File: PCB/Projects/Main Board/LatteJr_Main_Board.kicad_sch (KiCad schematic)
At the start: 134 parts, among them IC1 BQ27621YZFR-G1A, J1 Conn_01x04_Pin, J3 USB4056-03-A, J4 Conn_01x04_Pin, J5 Conn_01x04_Pin, J6 Conn_01x02_Socket, P1 RPI-RM2, Q1 BSS138DW, Q2 BSS138DW, SW1 SW_Push, SW2 SW_Push, SW3 SW_Push, SW4 SW_Push, SW5 SW_Push, SW6 SW_Push, SW7 SW_Push, SW8 SW_Push, U1 RP2350_60QFN, U10 HAL4395, U11 HAL4395, U12 HAL4395, U13 HAL4395, U14 HAL4395, U15 HAL4395, U16 HAL4395, U2 HAL4395, U3 HAL4395, U4 TPS63001DRCR, U5 BQ25180, U6 USBLC6-2P6, U7 USBLC6-2P6, U8 USBLC6-2P6, U9 HAL4395, Y1 ABM8-272-T3

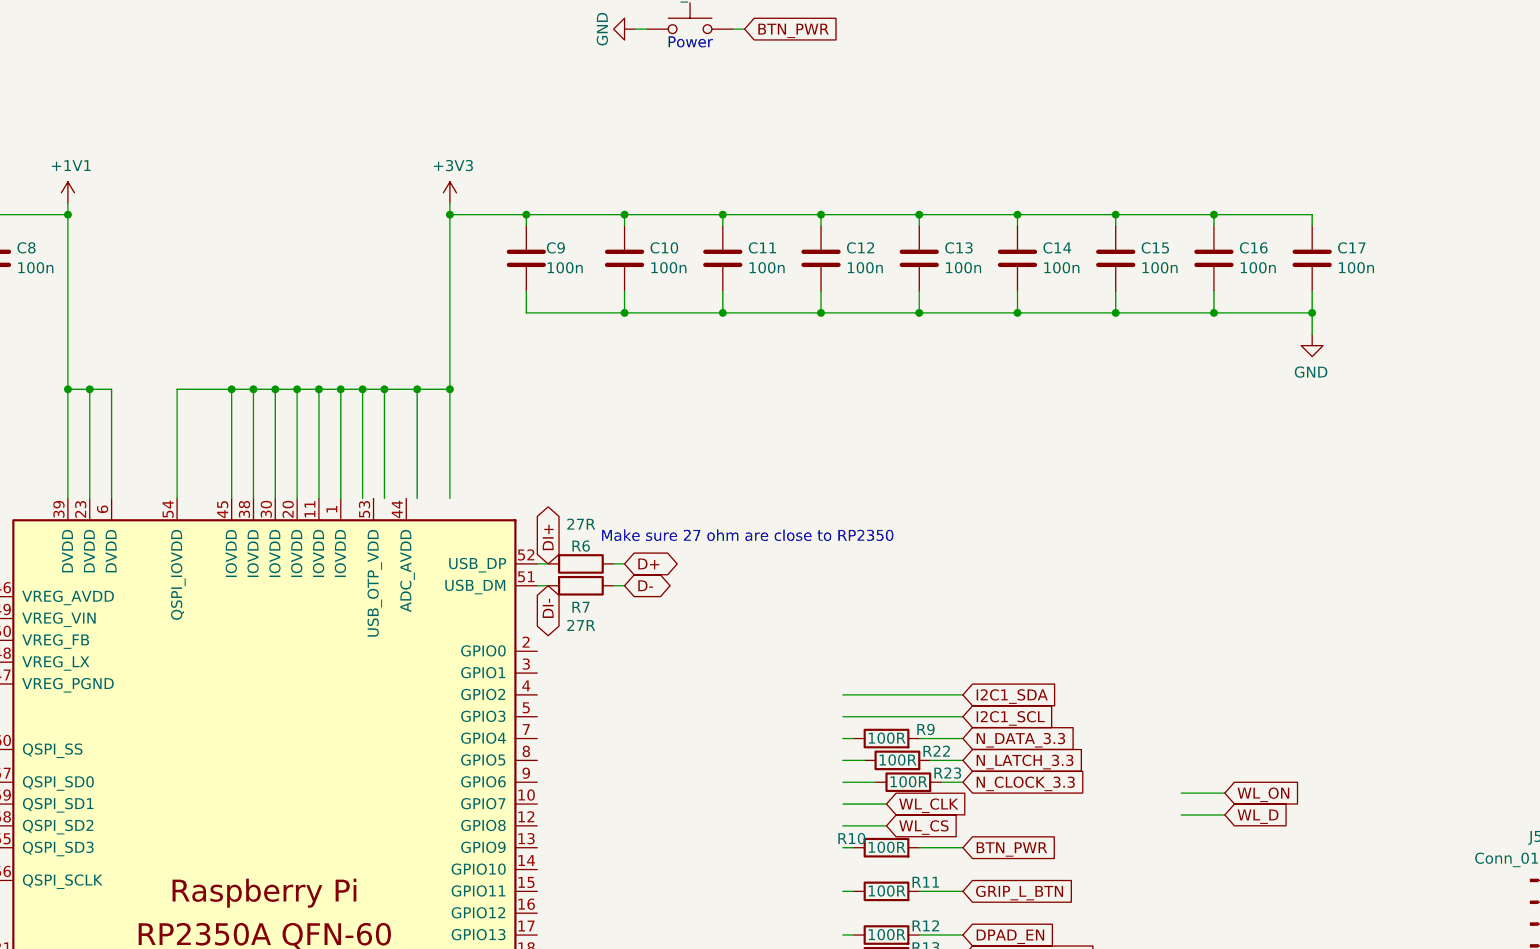
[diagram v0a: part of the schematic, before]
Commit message: Some Routing
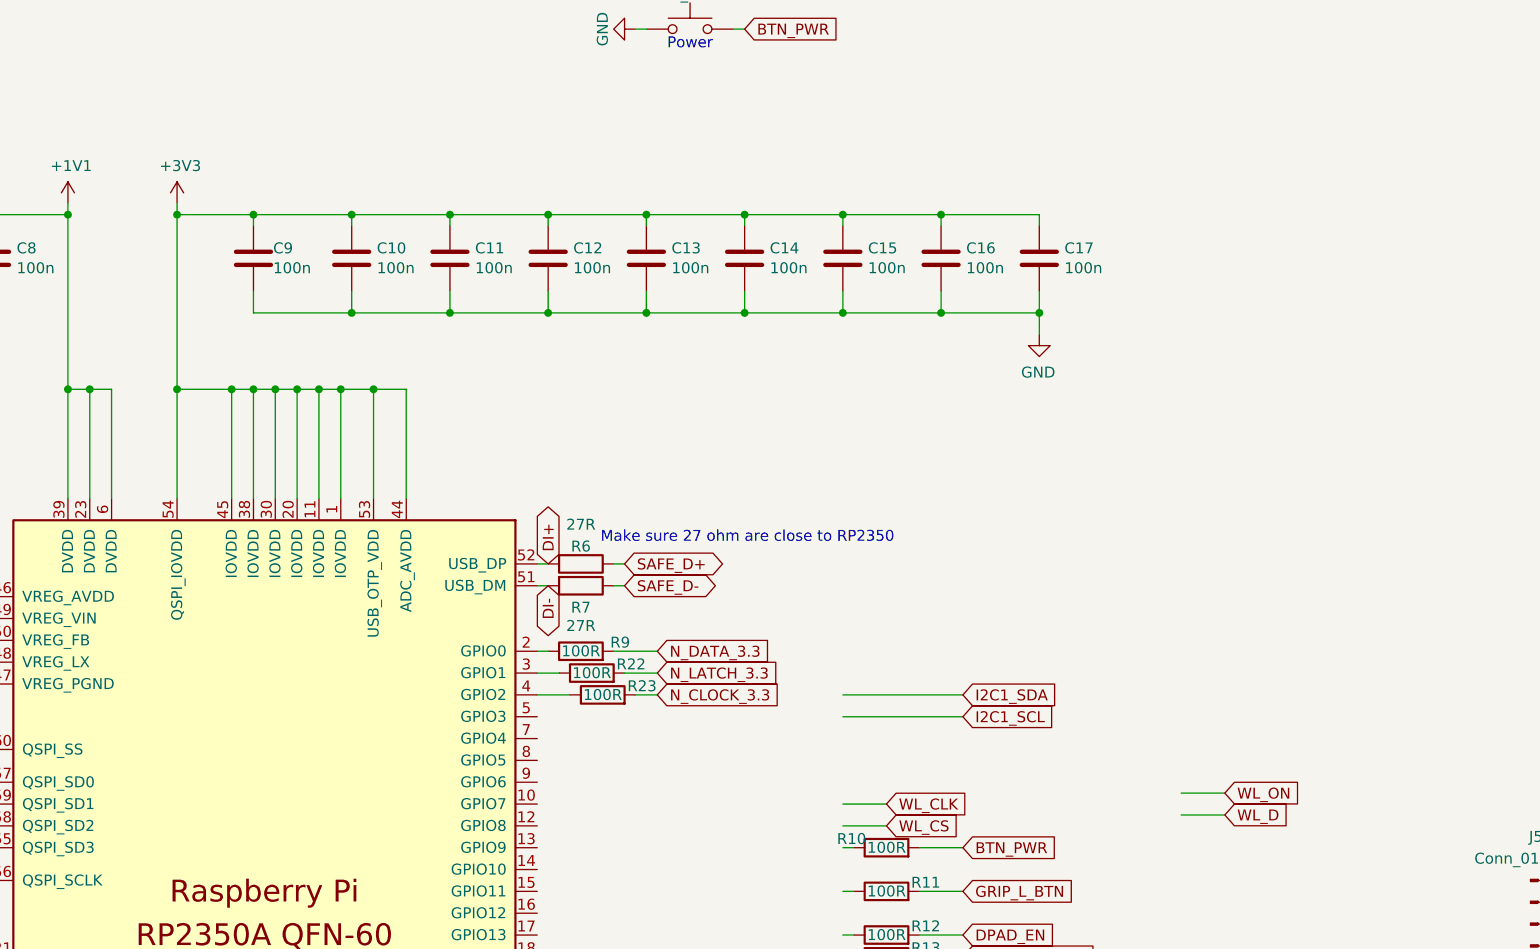
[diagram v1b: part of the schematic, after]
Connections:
- net +3V3: now also U1.44 (ADC_AVDD), U1.53 (USB_OTP_VDD)
- net D+: no longer R6.1
- net D-: no longer R7.1
- net SAFE_D+: now also R6.1
- net SAFE_D-: now also R7.1
- net at R22.1: now also U1.3 (GPIO1)
- net at R23.1: now also U1.4 (GPIO2)
- net at U1.2 (GPIO0): now also R9.1
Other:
- moved on the sheet: C10, C11, C12, C13, C14, C15, C16, C17, C9, R22, R23, R9
